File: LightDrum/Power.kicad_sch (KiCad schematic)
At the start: 67 parts, among them U1001 AP3401, U1002 LM22673-SOIC, U701 INA4181 A2, U702 INA4181 A2, U901 74HC2G08

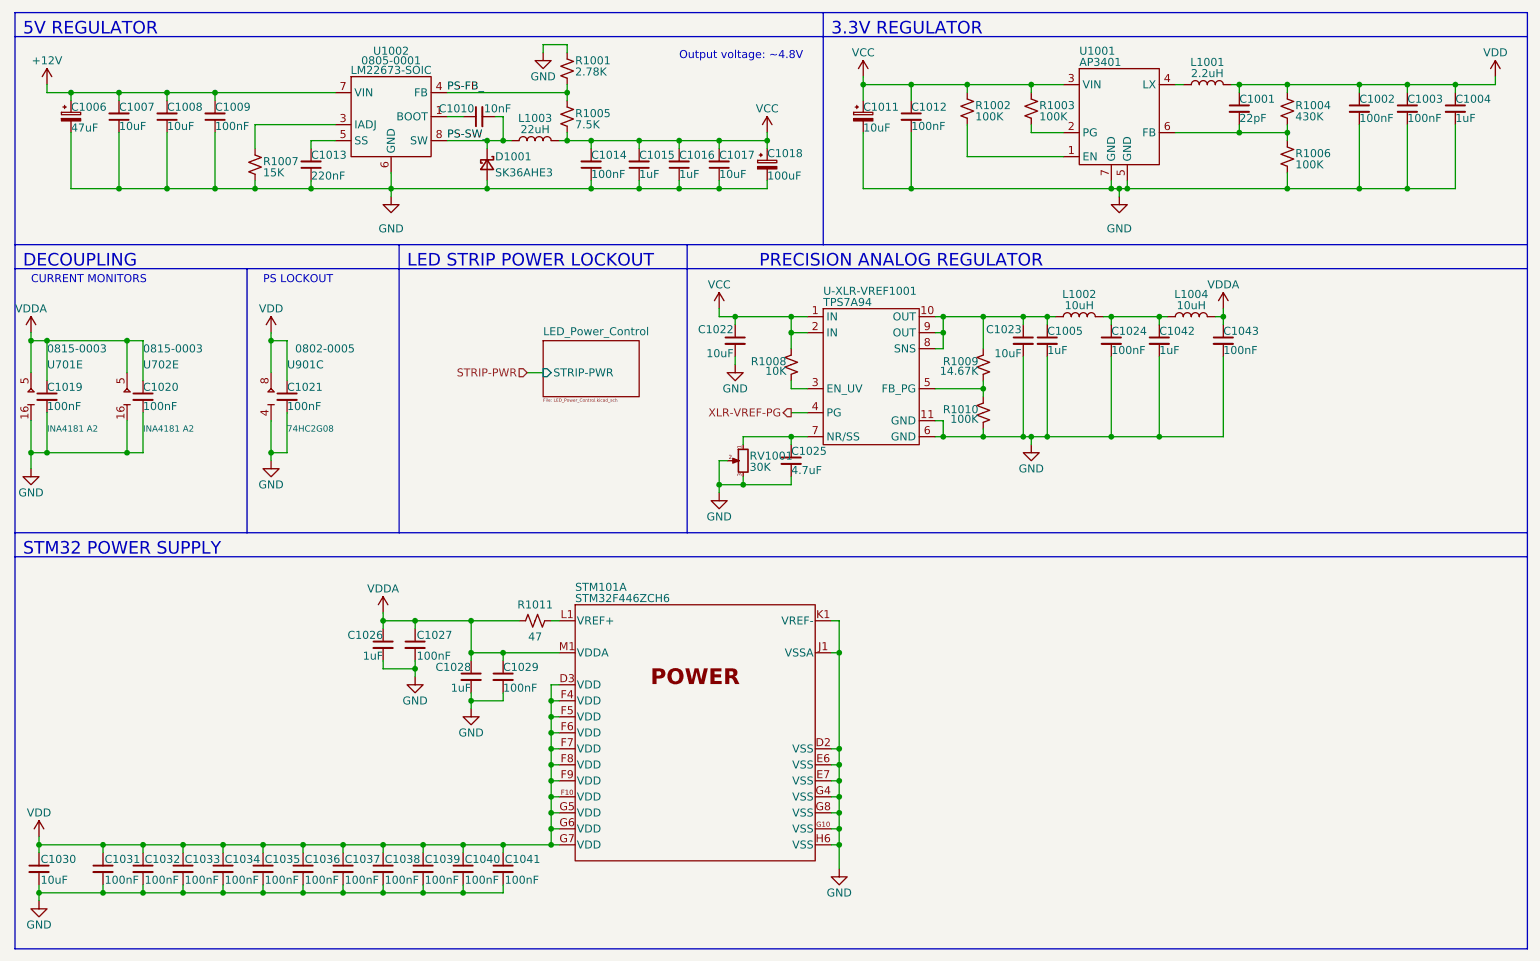
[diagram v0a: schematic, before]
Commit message: Lock REV8 Layout and send to PCB MNF
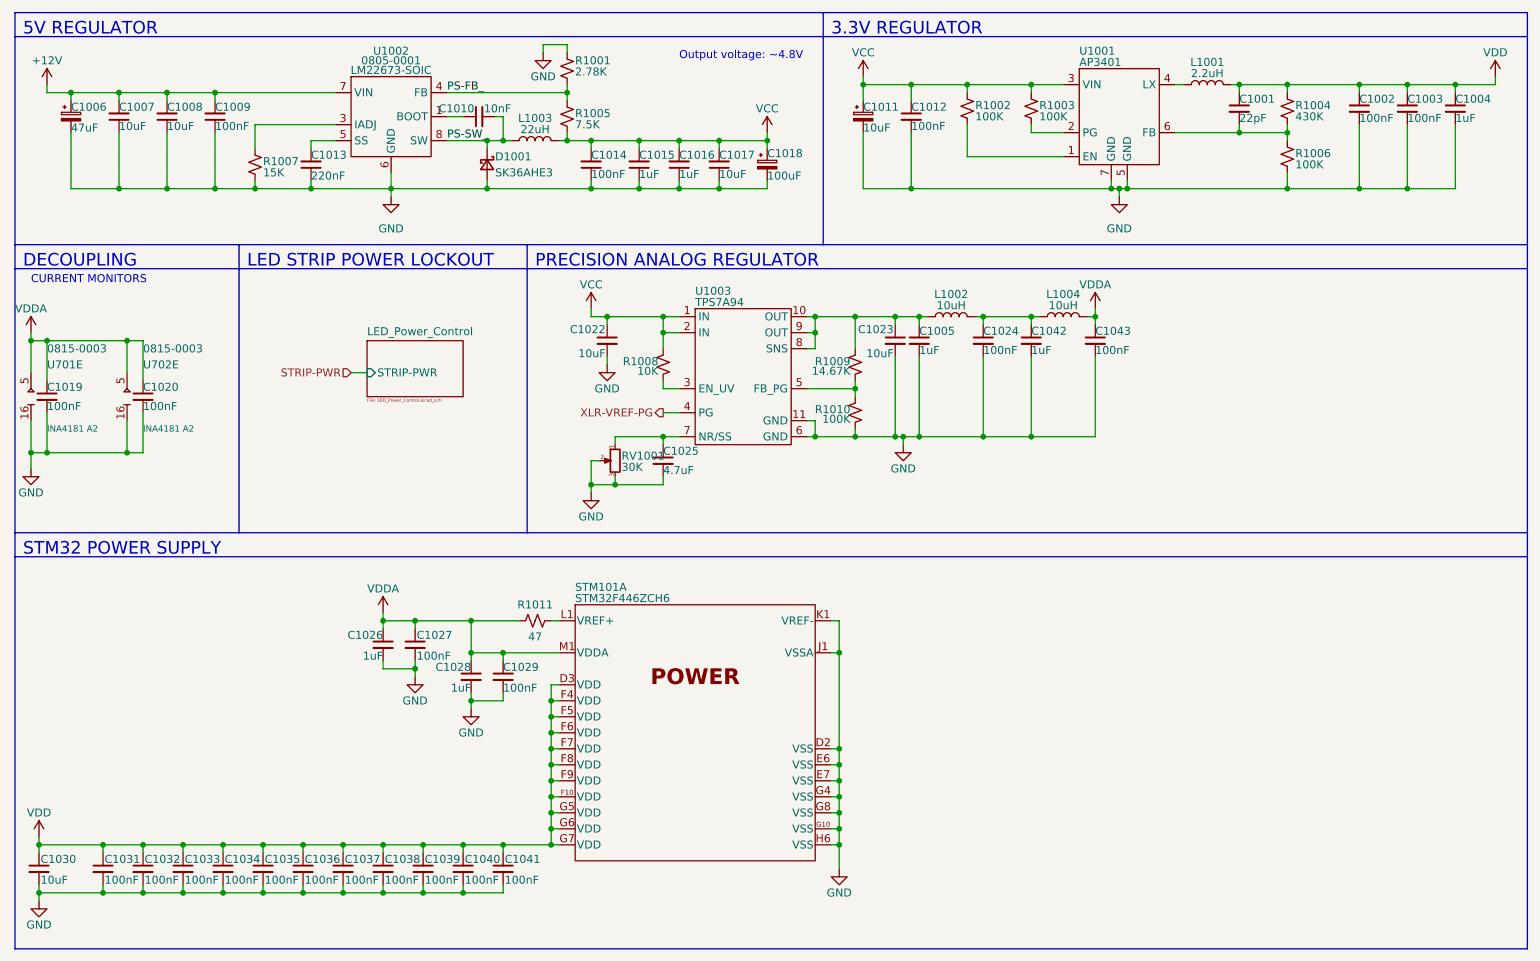
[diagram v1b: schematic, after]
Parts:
- removed C1021: 100nF, Capacitor_SMD:C_0603_1608Metric, symbol Device:C_Small
- removed U901: 74HC2G08, Package_SO:TSSOP-8_3x3mm_P0.65mm, symbol Daxxn_Logic:74HCT2G08
- renumbered U-XLR-VREF1001 to U1003
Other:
- note removed: "PS LOCKOUT"
- moved on the sheet: C1005, C1022, C1023, C1024, C1025, C1042, C1043, L1002, L1004, R1008, R1009, R1010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
